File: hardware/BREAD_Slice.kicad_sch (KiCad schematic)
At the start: 15 parts, among them J1 Conn_01x10_Female, J2 I2C_01x04

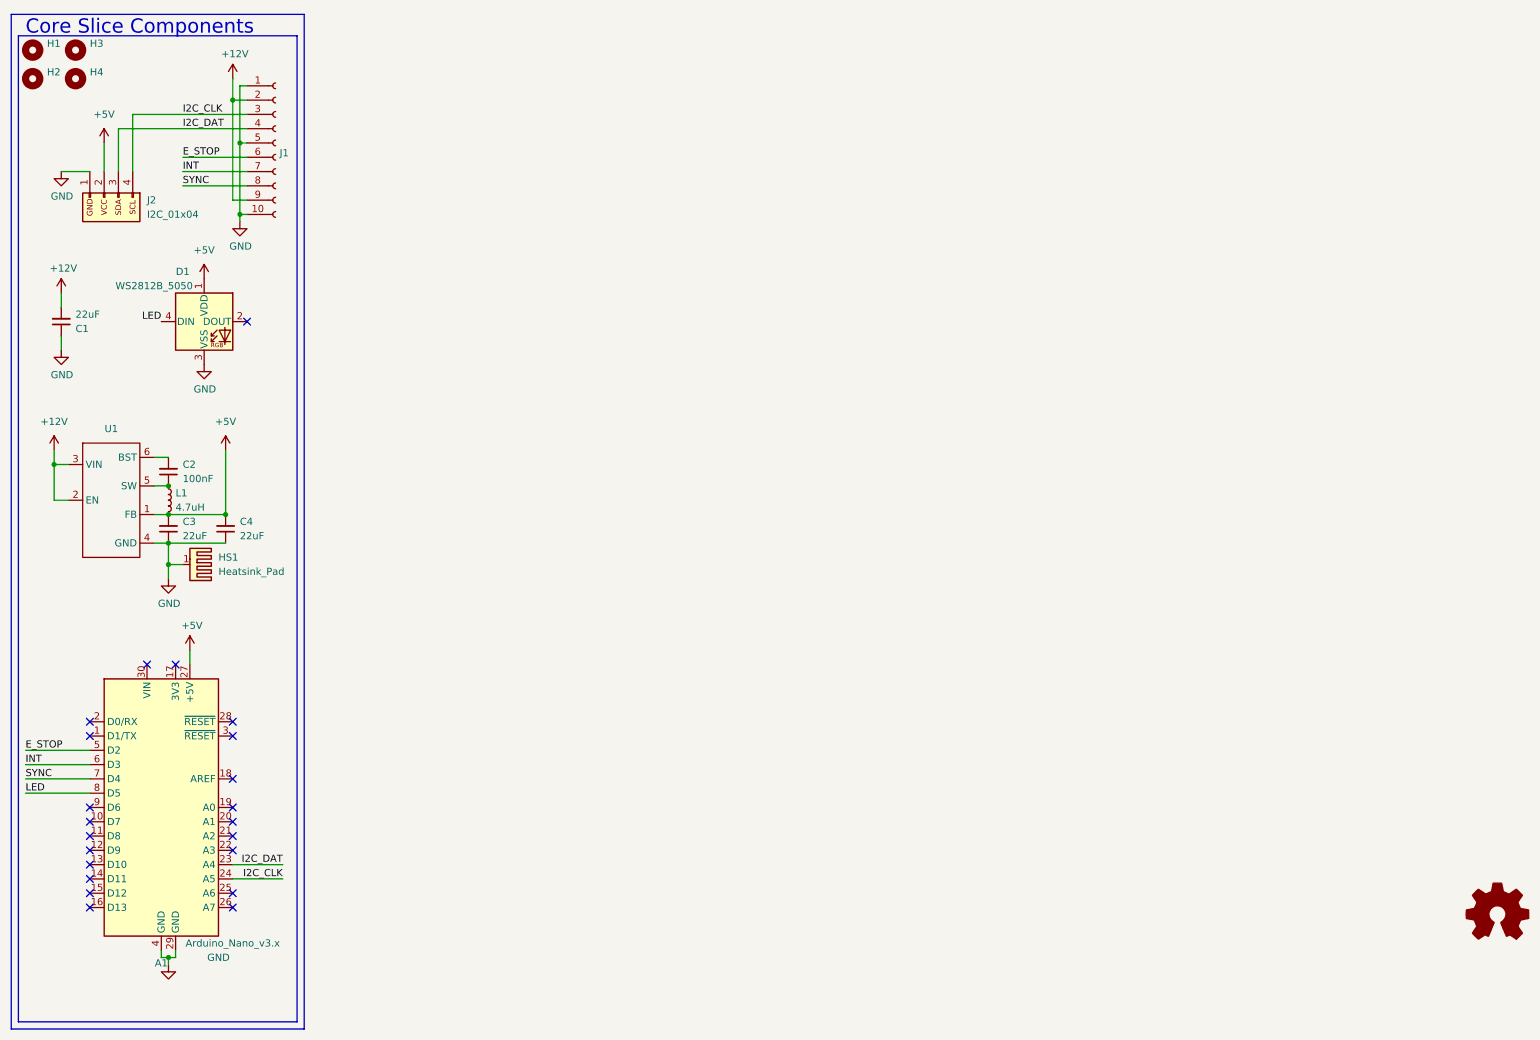
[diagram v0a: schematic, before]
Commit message: Initial commit
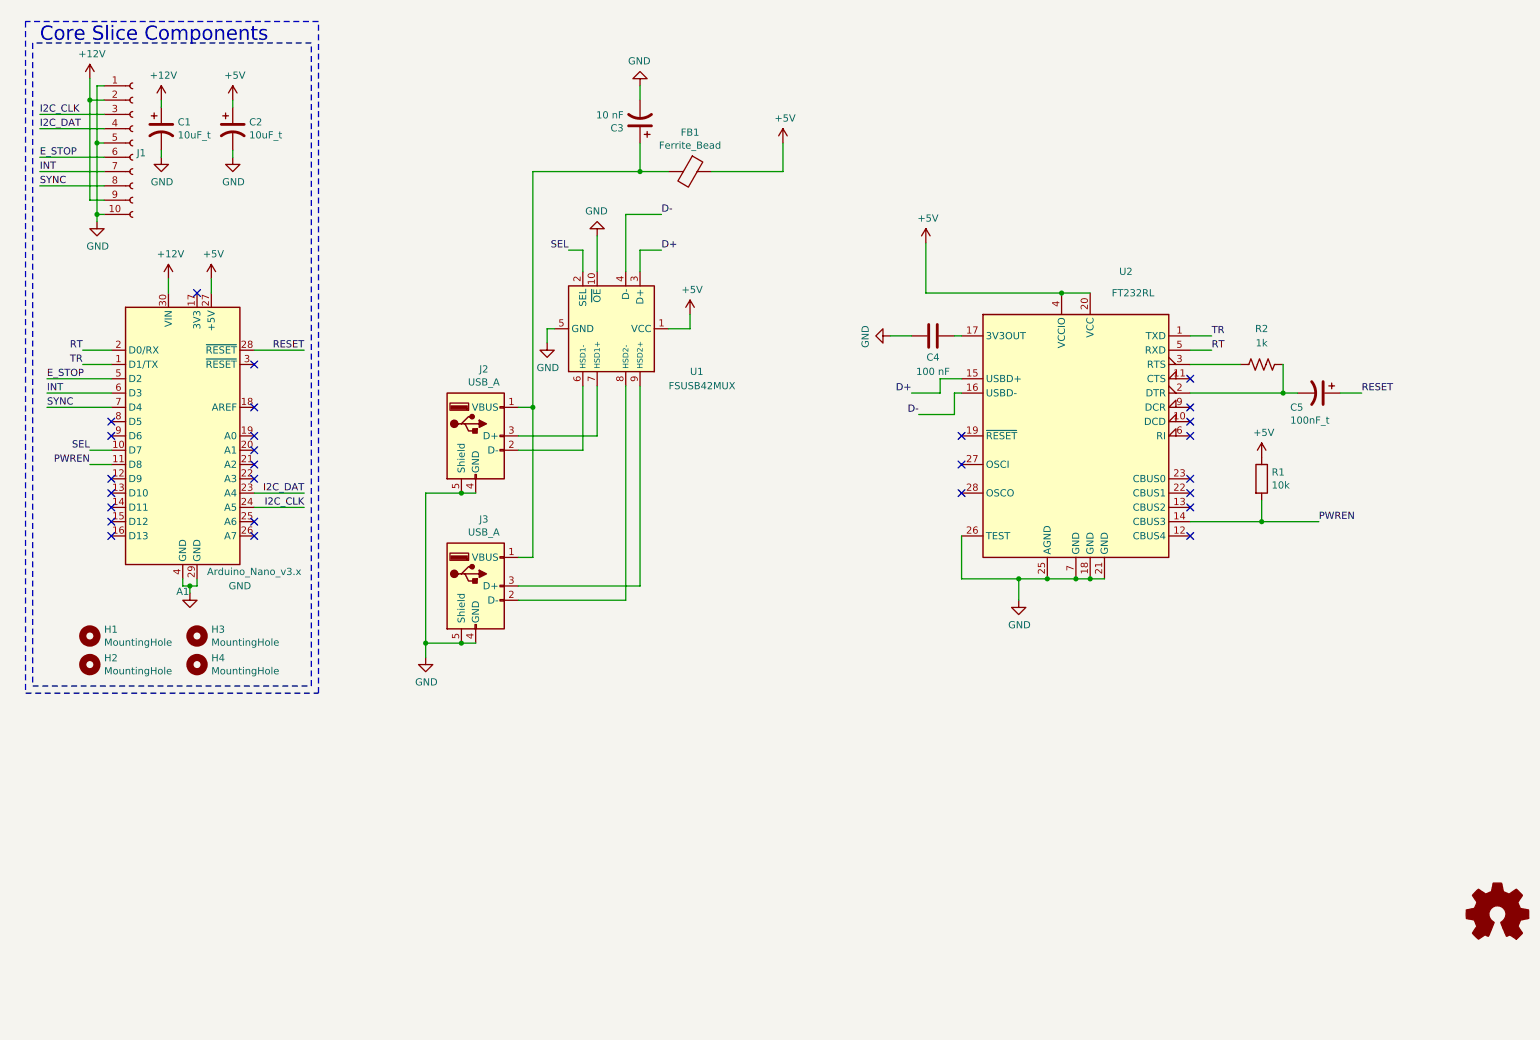
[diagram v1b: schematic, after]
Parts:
- removed C1, C3, C4: 22uF, Capacitor_SMD:C_1206_3216Metric, symbol Device:C_Small
- removed C2: 100nF, Capacitor_SMD:C_1206_3216Metric, symbol Device:C_Small
- removed D1: WS2812B_5050, SparkFun-LED:WS2812-5050-4PIN, symbol SparkFun-LED:WS2812B_5050
- removed HS1: Heatsink_Pad, SparkFun-Fuse:Thermal Pad, symbol Mechanical:Heatsink_Pad
- removed J2: I2C_01x04, Connector_JST:JST_SH_SM04B-SRSS-TB_1x04-1MP_P1.00mm_Horizontal, symbol SparkFun-Connector:I2C_01x04
- removed L1: 4.7uH, Inductor_SMD:L_1210_3225Metric, symbol Device:L_Small
- removed U1: ~, Package_TO_SOT_SMD:TSOT-23-6, symbol SparkFun-DiscreteSemi:AP63205
- added C1, C2: 10uF_t, OCI_UPL_FOOTPRINTS:C_2312, symbol BREAD_Slice-rescue:10uF_t-OCI_UPL_2_Capacitors-BREAD_Slice-rescue
- added C3: 10 nF, OCI_UPL_FOOTPRINTS:C_2312, symbol BREAD_Slice-rescue:10uF_t-OCI_UPL_2_Capacitors-BREAD_Slice-rescue
- added C4: 100 nF, Capacitor_SMD:C_1206_3216Metric_Pad1.33x1.80mm_HandSolder, symbol Device:C
- added C5: 100nF_t, Capacitor_SMD:C_1206_3216Metric_Pad1.33x1.80mm_HandSolder, symbol BREAD_Slice-rescue:10uF_t-OCI_UPL_2_Capacitors-BREAD_Slice-rescue
- added FB1: Ferrite_Bead, OCI_UPL_FOOTPRINTS:R_1206_HandSoldering, symbol BREAD_Slice-rescue:Ferrite_Bead-Device
- added J2, J3: USB_A, Connector_USB:USB_A_Molex_67643_Horizontal, symbol Connector:USB_A
- added Logo1: Logo_Open_Hardware_Small, Symbol:OSHW-Symbol_6.7x6mm_SilkScreen, symbol Graphic:Logo_Open_Hardware_Small
- added R1: 10k, OCI_UPL_FOOTPRINTS:R_1206_HandSoldering, symbol Device:R
- added R2: 1k, Resistor_SMD:R_1206_3216Metric_Pad1.30x1.75mm_HandSolder, symbol Device:R_US
- added U1: FSUSB42MUX, Package_SO:MSOP-10_3x3mm_P0.5mm, symbol Interface_USB:FSUSB42MUX
- added U2: FT232RL, Package_SO:SSOP-28_5.3x10.2mm_P0.65mm, symbol Interface_USB:FT232RL
- H1, H4: footprint MountingHole:MountingHole_5mm -> MountingHole:MountingHole_3.2mm_M3_DIN965_Pad
- H2: renamed from H3; footprint MountingHole:MountingHole_5mm -> MountingHole:MountingHole_3.2mm_M3_DIN965_Pad
- H3: renamed from H2; footprint MountingHole:MountingHole_5mm -> MountingHole:MountingHole_3.2mm_M3_DIN965_Pad
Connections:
- net +12V: now also A1.30 (VIN), C1.1
- net +5V: now also C2.1, FB1.1, R1.1, U1.1 (VCC), U2.20 (VCC), U2.4 (VCCIO)
- net GND: now also C1.2, C2.2, C3.2, C4.1, J2.4 (GND), J2.5 (Shield), J3.4 (GND), J3.5 (Shield), U1.10 (~{OE}), U1.5 (GND), U2.18 (GND), U2.21 (GND), U2.25 (AGND), U2.26 (TEST), U2.7 (GND)
- net TR: now reaches A1.1 (D1/TX)
- net TR: now also U2.1 (TXD)
- net SEL: now reaches A1.10 (D7)
- net SEL: now also U1.2 (SEL)
- net PWREN: now reaches A1.11 (D8)
- net PWREN: now also R1.2, U2.14 (CBUS3)
- net RT: now reaches A1.2 (D0/RX)
- net RT: now also U2.5 (RXD)
- net RESET: now reaches A1.28 (~{RESET})
- net RESET: now also C5.1
- net LED: no longer names the net of A1.8 (D5)
- new net: C3.1, FB1.2, J2.1 (VBUS), J3.1 (VBUS)
- new net: J3.2 (D-), U1.8 (HSD2-)
- new net: J3.3 (D+), U1.9 (HSD2+)
- new net: C4.2, U2.17 (3V3OUT)
- new net: C5.2, R2.2, U2.2 (DTR)
- new net: R2.1, U2.3 (RTS)
- new net: J2.2 (D-), U1.6 (HSD1-)
- new net: J2.3 (D+), U1.7 (HSD1+)
- new net D+: U1.3 (D+), U2.15 (USBD+)
- new net D-: U1.4 (D-), U2.16 (USBD-)
- no-connect marks 22 -> 27
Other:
- moved on the sheet: A1, H1, H2, H3, H4, J1
